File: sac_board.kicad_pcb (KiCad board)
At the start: 2 copper layers, 120 x 80 mm, 246 parts, among them J1 12V_Input, J2 USB_B_Mini, J3 Micro_SD_Card_Det1, J4 ARM JTAG/SWD, J5 DE9_Socket, J6 Conn_02x16_Odd_Even, J7 Conn_02x09_Odd_Even, J8 Conn_02x14_Odd_Even, J9 RJ45, U1 TPS563201, U10 TPS563201, U11 STM32F407VETx, U12 MAX3232, U13 LAN8742A, U2 TPS563201, U3 TPS563201, U4 TPS563201, U5 TPS563201, U6 TPS563201, U7 TPS563201, U8 TPS563201, U9 TPS563201, Y1 8MHz, Y2 32.768KHz, Y3 25MHz

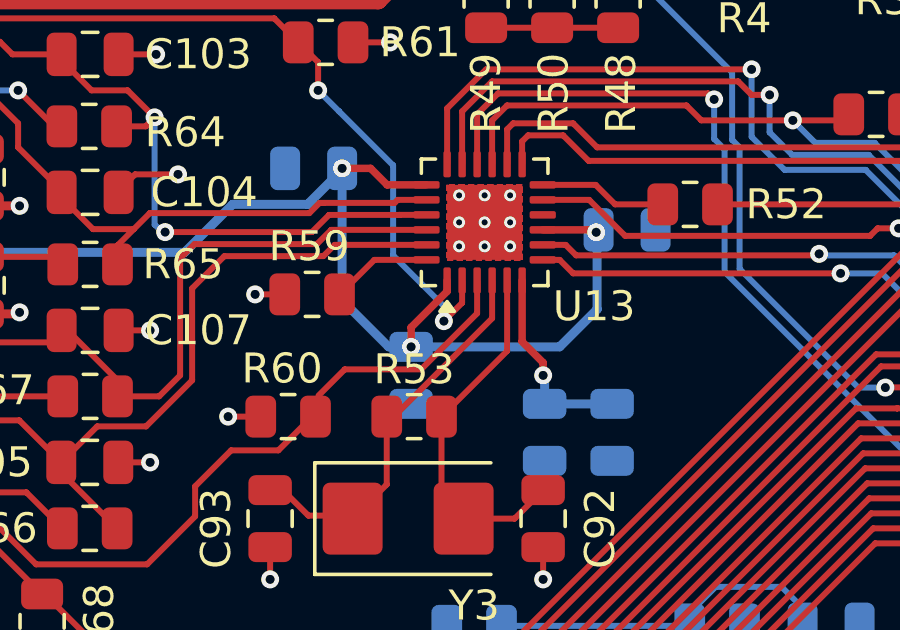
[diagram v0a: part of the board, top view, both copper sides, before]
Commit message: update
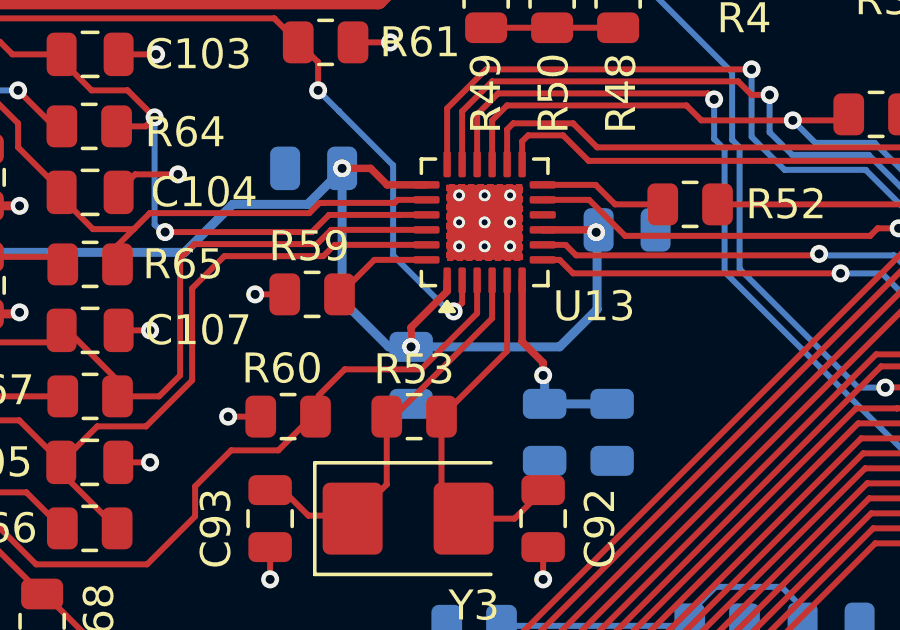
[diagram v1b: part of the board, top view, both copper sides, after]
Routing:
- net /mcu/LED-SPEED: track 45.8 -> 45.1 mm
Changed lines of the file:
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@@
-	)
-	(segment
-		(start 80 76.683884)
-		(end 80 75.9375)
-		(width 0.2)
-		(layer "F.Cu")
-		(net 131)
 	)
 	(segment
@@
 	)
 	(segment
+		(start 79.716942 76.966942)
+		(end 80 76.683884)
+		(width 0.2)
+		(layer "F.Cu")
+		(net 131)
+	)
+	(segment
+		(start 80 76.683884)
+		(end 80 75.9375)
+		(width 0.2)
+		(layer "F.Cu")
+		(net 131)
+	)
+	(segment
 		(start 75.2 68.6625)
 		(end 74.5375 68)
@@
 		(start 49.135 62.25)
 		(end 54.25 62.25)
-		(width 0.2)
-		(layer "F.Cu")
-		(net 131)
-	)
-	(segment
-		(start 79.391942 77.291942)
-		(end 80 76.683884)
 		(width 0.2)
 		(layer "F.Cu")
@@
 	)
 	(via
-		(at 79.391942 77.291942)
+		(at 79.716942 76.966942)
 		(size 0.6)
 		(drill 0.3)
@@
 	)
 	(segment
-		(start 75.899943 70.3)
-		(end 75.899943 70.299943)
-		(width 0.2)
-		(layer "B.Cu")
-		(net 131)
-	)
-	(segment
-		(start 79.562947 77.120937)
+		(start 79.712947 76.962947)
 		(end 79.562947 76.962947)
 		(width 0.2)
@@
 	)
 	(segment
-		(start 79.562947 76.962947)
-		(end 77.7 75.1)
+		(start 77.7 75.1)
+		(end 77.7 72.100057)
 		(width 0.2)
 		(layer "B.Cu")
@@
 	)
 	(segment
-		(start 79.391942 77.291942)
-		(end 79.562947 77.120937)
+		(start 79.716942 76.966942)
+		(end 79.712947 76.962947)
 		(width 0.2)
 		(layer "B.Cu")
@@
 	)
 	(segment
-		(start 77.7 75.1)
-		(end 77.7 72.100057)
+		(start 75.899943 70.3)
+		(end 75.899943 70.299943)
 		(width 0.2)
 		(layer "B.Cu")
@@
 		(width 0.2)
 		(layer "B.Cu")
+		(net 131)
+	)
+	(segment
+		(start 79.562947 76.962947)
+		(end 77.7 75.1)
+		(width 0.2)
+		(layer "B.Cu")
